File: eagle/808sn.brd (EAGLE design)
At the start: 100 x 80 mm, 82 parts, among them IC1 TL072P, IC3 TL072P, Q1 2N3904, Q45 2N3904, Q46 2N3906, Q47 2N3904, Q48 2N3904, Q49 2N3904

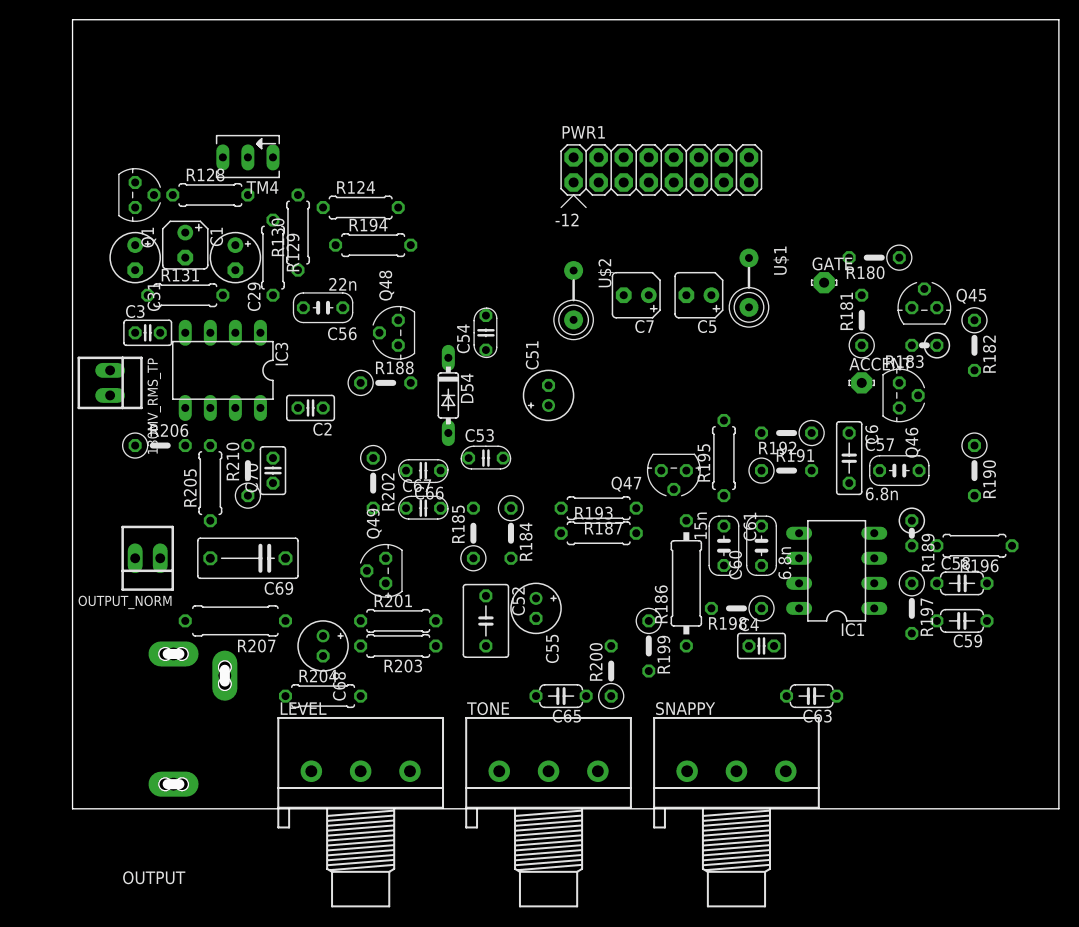
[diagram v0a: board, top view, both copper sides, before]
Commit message: routed
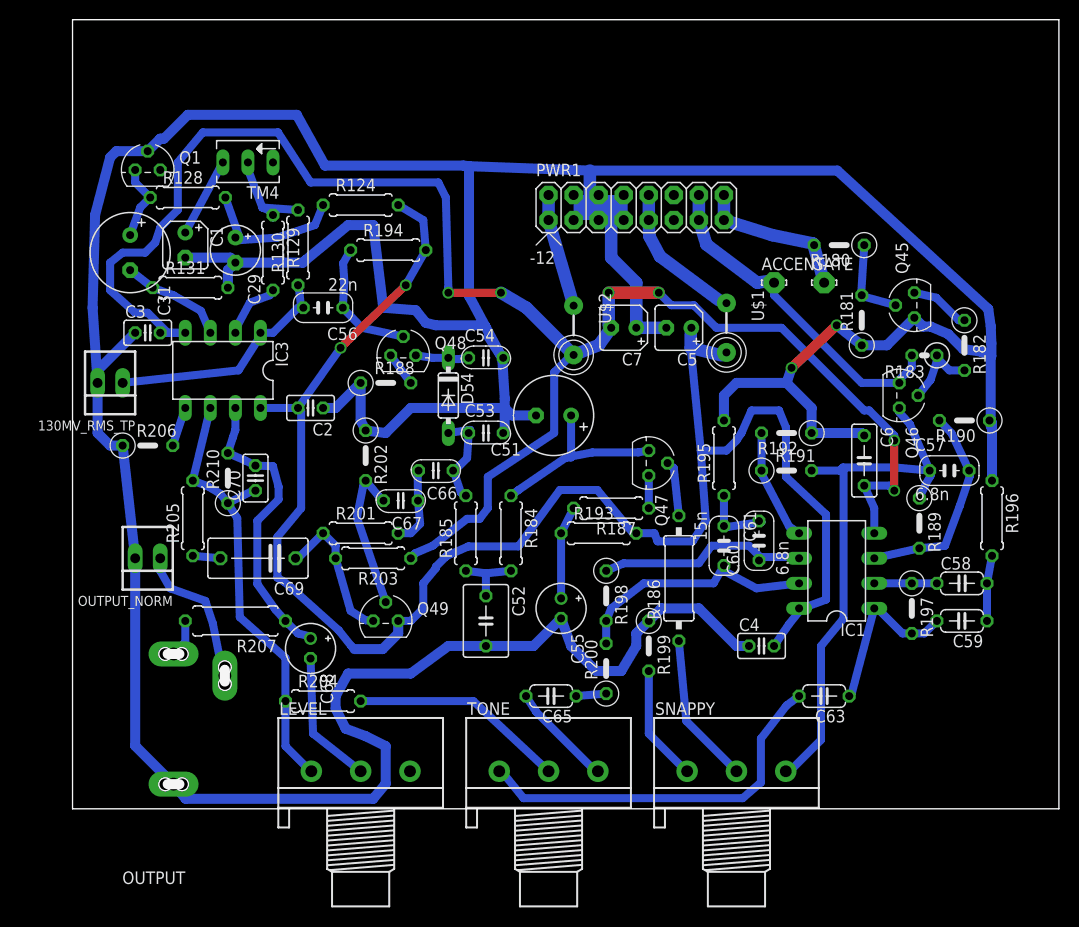
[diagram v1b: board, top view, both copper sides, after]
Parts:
- C31: device TR808clone:E2,5-5 -> TR808clone:E3,5-8
- C51: device TR808clone:E2-5 -> TR808clone:E3,5-8
- R184, R185: device TR808clone:0207/5V -> TR808clone:0207/7
- R189: device TR808clone:0207/2V -> TR808clone:0207/5V
- moved ACCENT 13.5 mm to (71.1, 53.3)
- moved R198 13.3 mm to (54.1, 21.6), turned to 270 degrees
- moved R201 9.67 mm to (29.2, 27.9)
- moved R203 9.25 mm to (30.5, 25.4)
- moved R190 5.18 mm to (90.4, 39.4), turned to 180 degrees
- moved U$1 5.11 mm to (66.3, 48.8)
- moved C57 5.08 mm to (88.9, 34.3)
- moved Q49 5.08 mm to (31.8, 19.1), turned to 0 degrees
- moved PWR1 4.58 mm to (54.6, 61.0)
- moved R205 3.98 mm to (12.2, 29.5)
- moved C5 3.88 mm to (61.5, 48.8)
- moved R180 3.78 mm to (77.7, 57.1)
- moved U$2 3.56 mm to (50.8, 48.5)
- moved C7 3.54 mm to (55.9, 48.8)
- moved R196 3.31 mm to (93.2, 29.5), turned to 270 degrees
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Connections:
- net GND: now also C5.-, C7.+, PWR1.3, PWR1.4, PWR1.5, PWR1.6, PWR1.7, PWR1.8
- net N$26: no longer C5.-, C7.+, PWR1.3, PWR1.4, PWR1.5, PWR1.6, PWR1.7, PWR1.8
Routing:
- net GND: track 0.00 -> 469.7 mm, vias 0 -> 2
- net -12V: track 0.00 -> 173.5 mm, vias 0 -> 6
- net +12V: track 0.00 -> 170.7 mm, vias 0 -> 2
- net N$9: track 0.00 -> 56.2 mm
- net N$35: track 0.00 -> 45.7 mm
- net N$17: track 0.00 -> 38.7 mm
- net TRIG: track 0.00 -> 34.7 mm
- net N$129: track 0.00 -> 30.4 mm
- net N$14: track 0.00 -> 25.6 mm
- net WN1: track 0.00 -> 24.0 mm
- net N$34: track 0.00 -> 21.9 mm
- net N$160: track 0.00 -> 21.7 mm
- net N$8: track 0.00 -> 21.3 mm
- net N$26: track 0.00 -> 20.0 mm
- net N$12: track 0.00 -> 17.2 mm
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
